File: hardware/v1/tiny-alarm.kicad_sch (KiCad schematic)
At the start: 66 parts, among them J1 Battery, J2 USB_C_Receptacle_USB2.0_16P, J3 ISP_HEADER, J4 Touch_Sensor, J5 SSD_1306_OLED, Q1 SS8050, SW1 SW_SPDT, SW2 SW_Push, SW3 SW_Push, SW4 SW_Push, SW5 SW_Push, SW6 SW_Push, U1 MT3608, U2 TP4056-42-ESOP8, U3 USBLC6-2SC6, U4 CH340C, U5 ATmega328P-A, U6 DS3231SN, Y1 16MHZ

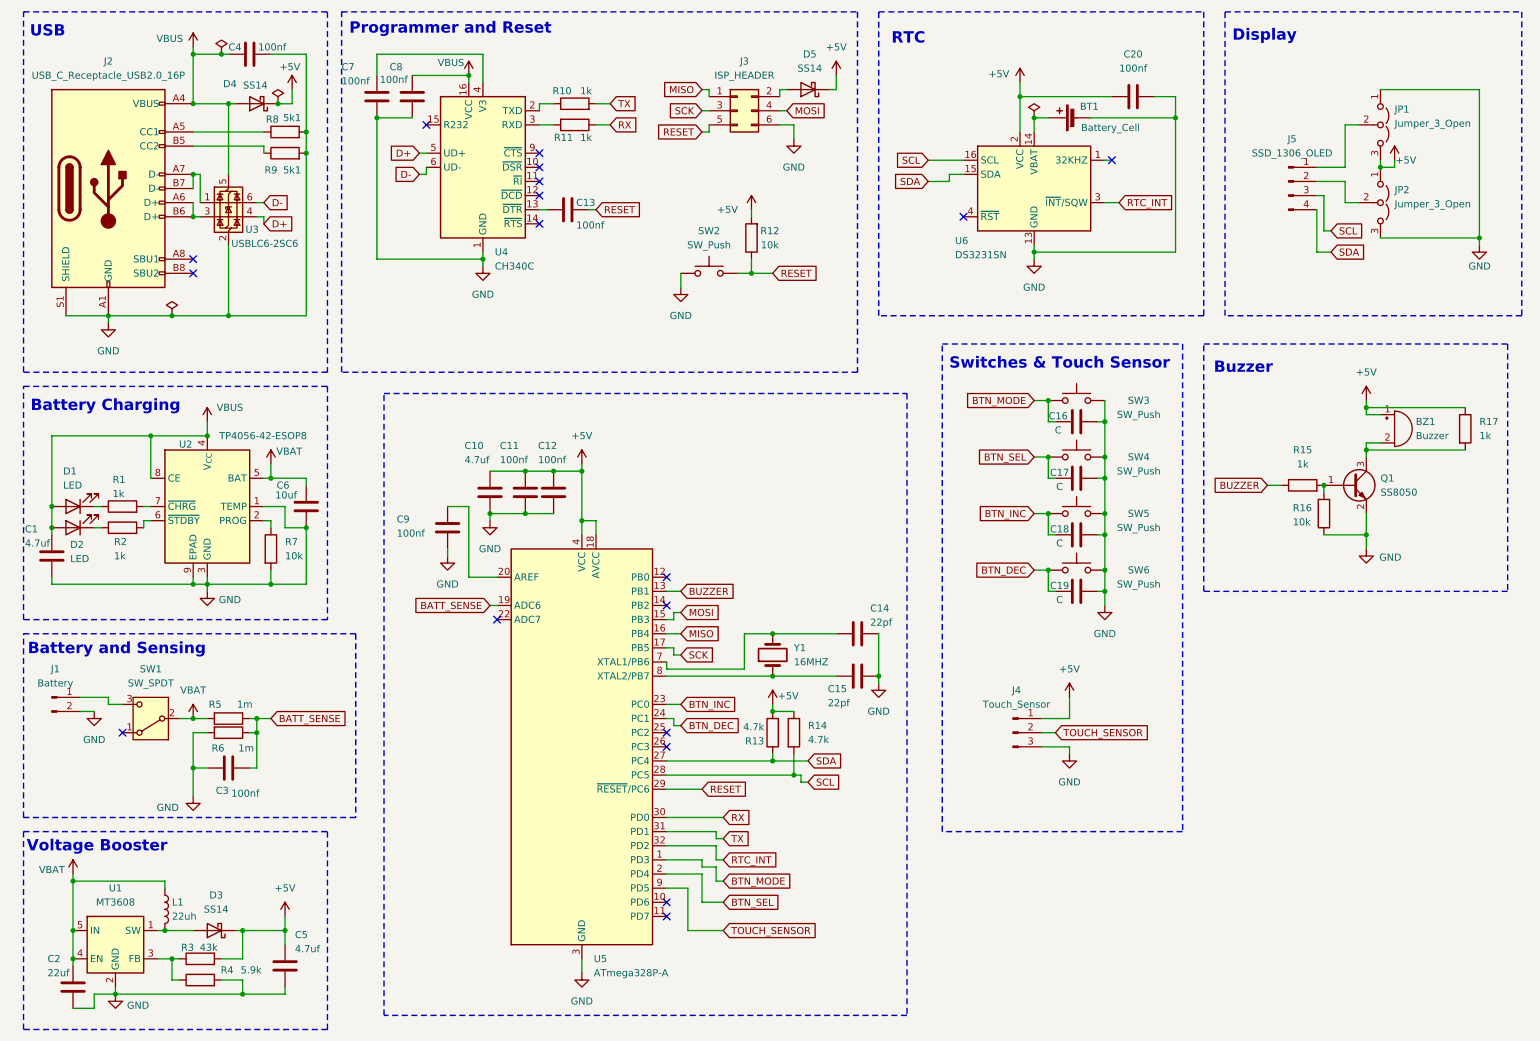
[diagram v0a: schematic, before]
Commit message: fix: more schematic fixes
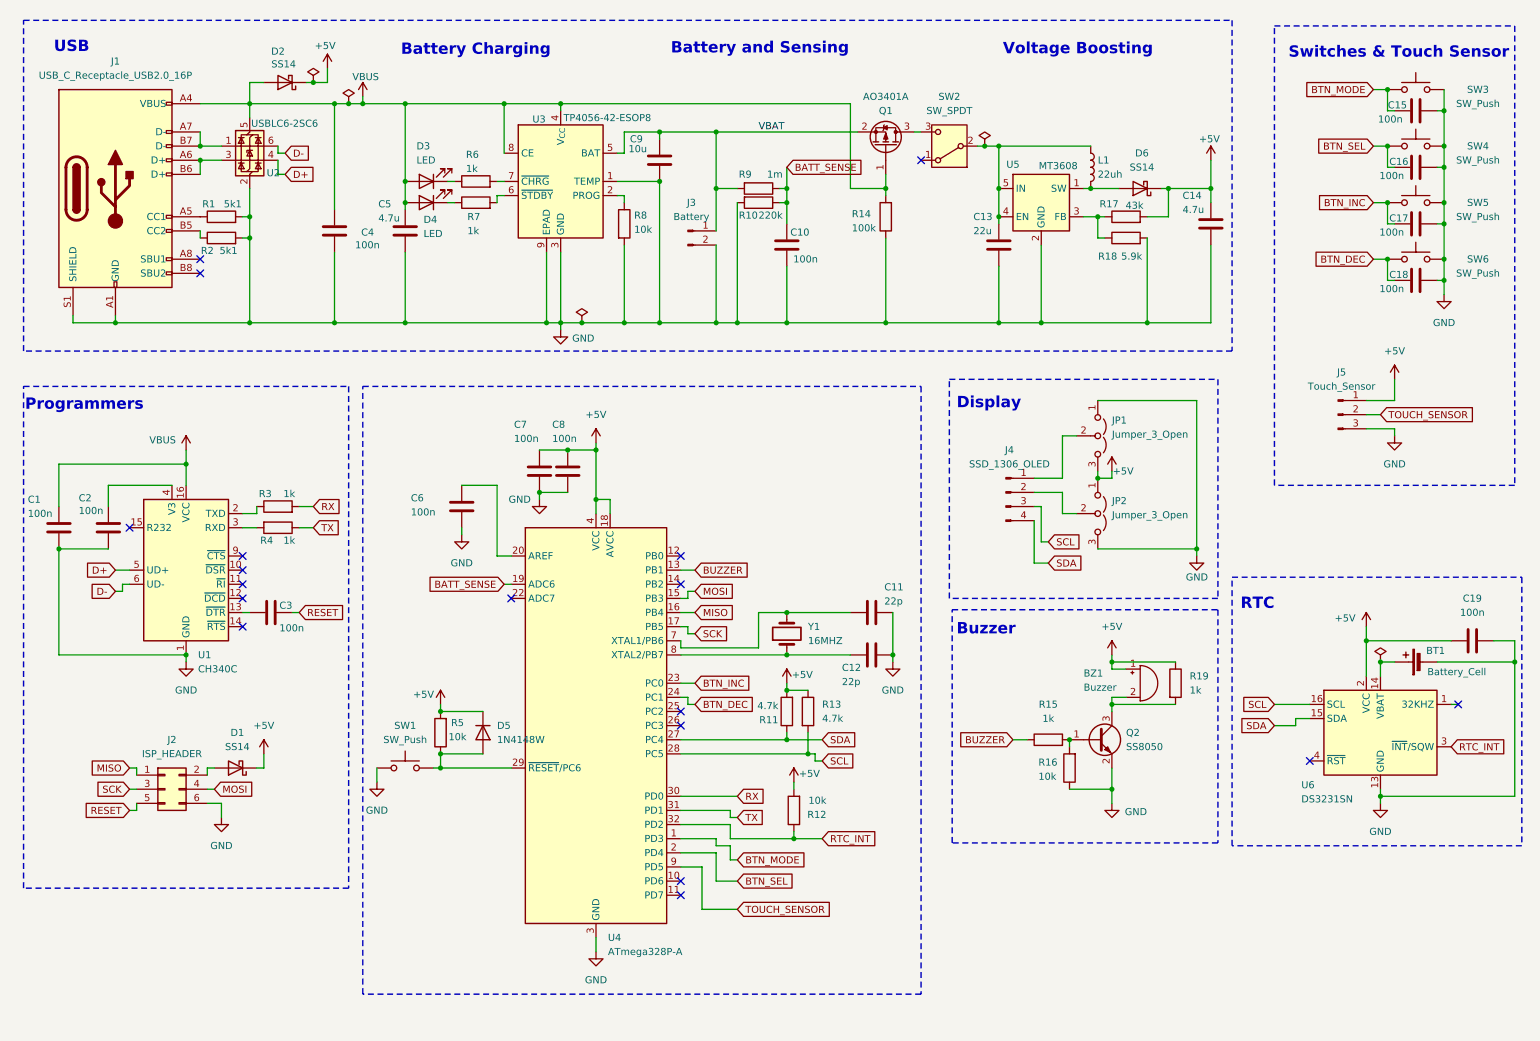
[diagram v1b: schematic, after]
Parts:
- removed C6: 10uf, symbol Device:C
- removed C7, C8: 100nf, symbol Device:C
- removed D1, D2: LED, symbol Device:LED
- removed D3, D4: SS14, Diode_SMD:D_SMA, symbol Diode:SS14
- removed J1: Battery, symbol Connector:Conn_01x02_Pin
- removed J2: USB_C_Receptacle_USB2.0_16P, symbol Connector:USB_C_Receptacle_USB2.0_16P
- removed R11: 1k, symbol Device:R
- removed R5: 1m, symbol Device:R
- removed SW1: SW_SPDT, symbol Switch:SW_SPDT
- removed U1: MT3608, Package_TO_SOT_SMD:SOT-23-6, symbol Regulator_Switching:MT3608
- removed U2: TP4056-42-ESOP8, Package_SO:SOIC-8-1EP_3.9x4.9mm_P1.27mm_EP2.41x3.3mm_ThermalVias, symbol Battery_Management:TP4056-42-ESOP8
- removed U3: USBLC6-2SC6, Package_TO_SOT_SMD:SOT-23-6, symbol Power_Protection:USBLC6-2SC6
- removed U4: CH340C, Package_SO:SOIC-16_3.9x9.9mm_P1.27mm, symbol Interface_USB:CH340C
- added C14: 4.7u, symbol Device:C
- added C9: 10u, symbol Device:C
- added D2, D6: SS14, Diode_SMD:D_SMA, symbol Diode:SS14
- added D3, D4: LED, symbol Device:LED
- added D5: 1N4148W, Diode_SMD:D_SOD-123, symbol Diode:1N4148W
- added J1: USB_C_Receptacle_USB2.0_16P, symbol tiny-alarm:USB_C_Receptacle_USB2.0_16P
- added J3: Battery, symbol Connector:Conn_01x02_Pin
- added Q1: AO3401A, Package_TO_SOT_SMD:SOT-23, symbol Transistor_FET:AO3401A
- added R12: 10k, symbol Device:R
- added R14: 100k, symbol Device:R
- added R17: 43k, symbol Device:R
- added R18: 5.9k, symbol Device:R
- added SW2: SW_SPDT, symbol Switch:SW_SPDT
- added U1: CH340C, Package_SO:SOIC-16_3.9x9.9mm_P1.27mm, symbol tiny-alarm:CH340C
- added U2: USBLC6-2SC6, Package_TO_SOT_SMD:SOT-23-6, symbol Power_Protection:USBLC6-2SC6
- added U3: TP4056-42-ESOP8, Package_SO:SOIC-8-1EP_3.9x4.9mm_P1.27mm_EP2.41x3.3mm_ThermalVias, symbol Battery_Management:TP4056-42-ESOP8
- added U5: MT3608, Package_TO_SOT_SMD:SOT-23-6, symbol Regulator_Switching:MT3608
- C1, C10: value 4.7uf -> 100n
- C11: renamed from C14; value 22pf -> 22p
- C12: renamed from C15; value 22pf -> 22p
- C13: value 100nf -> 22u
- C15: renamed from C16; value C -> 100n
- C16: renamed from C17; value C -> 100n
- C17: renamed from C18; value C -> 100n
- C18: renamed from C19; value C -> 100n
- C19: renamed from C20; value 100nf -> 100n
- C2: value 22uf -> 100n
- C3, C4: value 100nf -> 100n
- C5: value 4.7uf -> 4.7u
- C6: renamed from C9; value 100nf -> 100n
- C7: renamed from C11; value 100nf -> 100n
- C8: renamed from C12; value 100nf -> 100n
- R1, R2: value 1k -> 5k1
- R10: value 1k -> 220k
- R3: value 43k -> 1k
- R4: value 5.9k -> 1k
- R6: value 1m -> 1k
- R7: value 10k -> 1k
- R8: value 5k1 -> 10k
- R9: value 5k1 -> 1m
- U4: renamed from U5; symbol MCU_Microchip_ATmega:ATmega328P-A -> tiny-alarm:ATmega328P-A
- renumbered D5 to D1, J3 to J2, J5 to J4, J4 to J5, Q1 to Q2, R13 to R11, R14 to R13, R17 to R19, R12 to R5, SW2 to SW1
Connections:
- net +5V: now also C14.1, D2.1 (K), D5.1 (K), D6.1 (K), R12.2, R17.2; no longer C10.1, C5.1, R3.2
- net BATT_SENSE: now also C10.1, R10.1, R9.1; no longer C3.1, R6.1
- net D+: now also U1.5 (UD+), U2.4 (I/O2)
- net D-: now also U1.6 (UD-), U2.6 (I/O1)
- net GND: now also C13.2, C4.1, R1.2, R10.2, R2.2, C14.2, C9.2, J1.A1 (GND), J1.A12 (GND), J1.B1 (GND), J1.B12 (GND), J1.S1 (SHIELD), J3.2 (Pin_2), R14.1, R18.2, U1.1 (GND), U2.2 (GND), U3.1 (TEMP), U3.3 (GND), U3.9 (EPAD), U5.2 (GND); no longer C3.2, C4.2, R4.2, R6.2, R7.2, R9.2
- net RESET: now also C3.1; no longer C13.1, R5.1, SW1.2, U4.29 (~{RESET}/PC6)
- net RTC_INT: now also R12.1
- net RX: now also R3.2
- net TX: now also R4.1; no longer R10.2
- net VBAT: now also R9.2, C9.1, J3.1 (Pin_1), Q1.2 (S), U3.5 (BAT); no longer C2.1, L1.1
- net VBUS: now also C4.2, C5.1, D2.2 (A), D3.2 (A), D4.2 (A), J1.A4 (VBUS), J1.A9 (VBUS), J1.B4 (VBUS), J1.B9 (VBUS), Q1.1 (G), R14.2, U1.16 (VCC), U2.5 (VBUS), U3.4 (V_{CC}), U3.8 (CE); no longer C4.1
- net at R2.1: now also J1.B5 (CC2)
- net at R1.1: now also J1.A5 (CC1)
- net at L1.2: now also D6.2 (A), U5.1 (SW)
- net at R8.1: now also U3.2 (PROG)
- net at R3.1: now also U1.2 (TXD); no longer R4.1
- net at R7.1: now also D4.1 (K)
- new net: D5.2 (A), R5.1, SW1.2, U4.29 (~{RESET}/PC6)
- new net: C3.2, U1.13 (~{DTR})
- new net: D3.1 (K), R6.1
- new net: R6.2, U3.7 (~{CHRG})
- new net: R7.2, U3.6 (~{STDBY})
- new net: C13.1, L1.1, SW2.2 (B), U5.4 (EN), U5.5 (IN)
- new net: Q1.3 (D), SW2.3 (C)
- new net: R17.1, R18.1, U5.3 (FB)
- new net: R4.2, U1.3 (RXD)
- new net: J1.A7 (D-), J1.B7 (D-), U2.1 (I/O1)
- new net: J1.A6 (D+), J1.B6 (D+), U2.3 (I/O2)
- new net: C2.1, U1.4 (V3)
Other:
- note added: "Programmers"
- note added: "Voltage Boosting"
- note removed: "Programmer and Reset"
- note removed: "Voltage Booster"
- moved on the sheet: BT1, BZ1, C11, C12, C15, C16, C17, C18, C19, C6, C7, C8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
